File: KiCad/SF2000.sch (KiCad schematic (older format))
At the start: 76 parts, among them J1 Conn_2Rows-86Pins_even_odd, J2 Conn_01x02, J7 Conn_02x01, U1 LM1117-3.3, U19 74LVC1G57GV, U2 ABLIC S-1132B43-M5T1U, U3 TLV75533PDBVR, U4 SN74CBT16211, U5 SN74CBT16211, U6 SN74CBT3244PW, U7 SN74LVC16245ADGGR

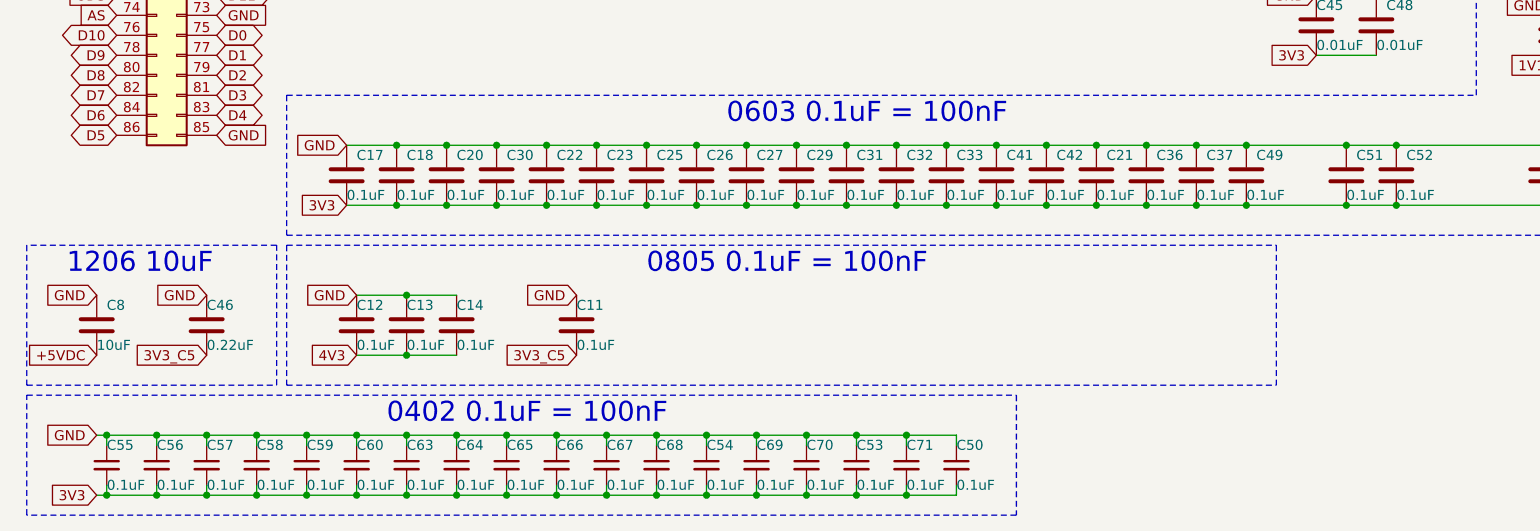
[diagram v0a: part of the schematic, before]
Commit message: Change C51 to size 0402
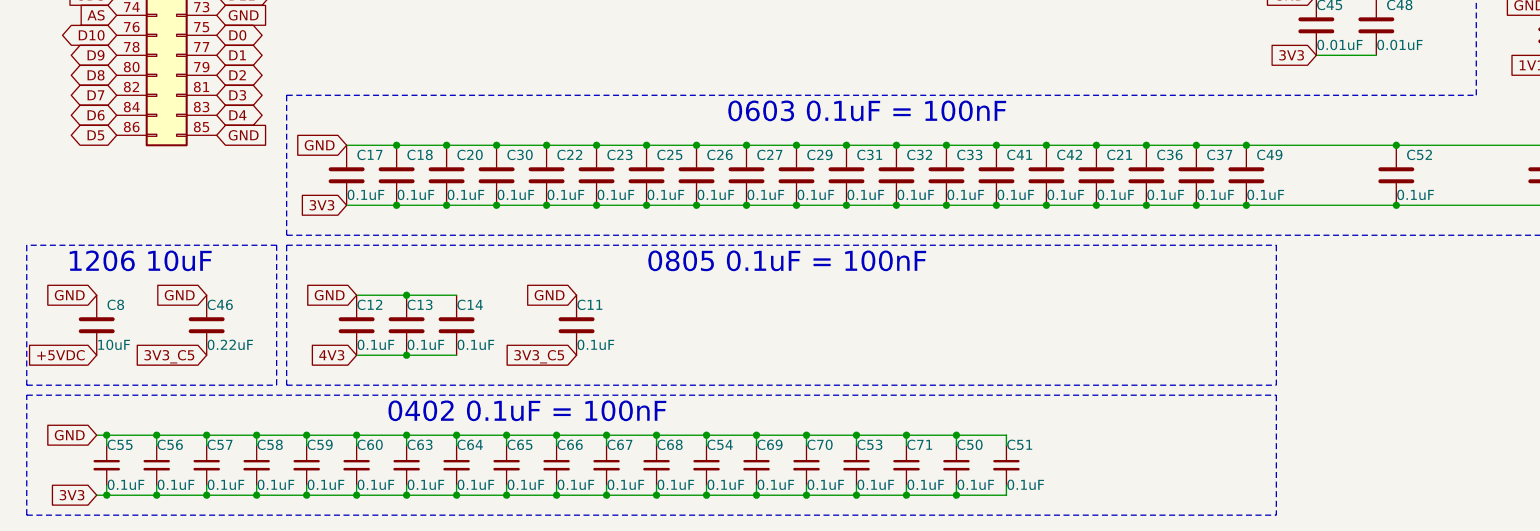
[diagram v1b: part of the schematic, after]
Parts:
- removed C51: 0.1uF, Capacitor_SMD:C_0603_1608Metric_Pad1.08x0.95mm_HandSolder, symbol Device:C
- added C51: 0.1uF, Capacitor_SMD:C_0402_1005Metric_Pad0.74x0.62mm_HandSolder, symbol Device:C_Small
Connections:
- net 3V3: now also C51.2
- net GND: now also C51.1
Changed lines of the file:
@@
-$EndComp
-$Comp
-L Device:C C51
-U 1 1 623684AD
-P 7150 6050
-F 0 "C51" H 7200 6150 50  0000 L CNN
-F 1 "0.1uF" H 7150 5950 50  0000 L CNN
-F 2 "Capacitor_SMD:C_0603_1608Metric_Pad1.08x0.95mm_HandSolder" H 7188 5900 50  0001 C CNN
-F 3 "~" H 7150 6050 50  0001 C CNN
-	1    7150 6050
-	1    0    0    -1
 $EndComp
 $Comp
@@
 Wire Notes Line
 	1850 6350 10000 6350
-Wire Wire Line
-	7400 5900 7150 5900
-Connection ~ 7150 5900
-Wire Wire Line
-	7400 6200 7150 6200
-Connection ~ 7150 6200
 Connection ~ 7400 5900
 Connection ~ 7400 6200
@@
 $EndComp
 Wire Notes Line
-	550  7150 5500 7150
-Wire Notes Line
-	5500 7150 5500 7750
-Wire Notes Line
-	5500 7750 550  7750
+	6800 7150 6800 7750
 Wire Notes Line
 	550  7750 550  7150
@@
 	5200 7650 4950 7650
 Connection ~ 4950 7650
-Wire Wire Line
-	6650 5900 7150 5900
-Wire Wire Line
-	6650 6200 7150 6200
+Wire Notes Line
+	550  7150 6800 7150
+Wire Notes Line
+	550  7750 6800 7750
+$Comp
+L Device:C_Small C51
+U 1 1 6BCECA9F
+P 5450 7500
+F 0 "C51" H 5450 7600 50  0000 L CNN
+F 1 "0.1uF" H 5450 7400 50  0000 L CNN
+F 2 "Capacitor_SMD:C_0402_1005Metric_Pad0.74x0.62mm_HandSolder" H 5450 7500 50  0001 C CNN
+F 3 "~" H 5450 7500 50  0001 C CNN
+	1    5450 7500
+	1    0    0    -1
+$EndComp
+Wire Wire Line
+	6650 5900 7400 5900
+Wire Wire Line
+	6650 6200 7400 6200
+Wire Wire Line
+	5200 7350 5450 7350
+Wire Wire Line
+	5450 7350 5450 7400
+Connection ~ 5200 7350
+Wire Wire Line
+	5200 7650 5450 7650
+Wire Wire Line
+	5450 7650 5450 7600
+Connection ~ 5200 7650
 $EndSCHEMATC
